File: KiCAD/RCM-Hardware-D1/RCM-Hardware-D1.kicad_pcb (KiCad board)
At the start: 2 copper layers, 66 x 63.5 mm, 2 parts, among them U1 WeMos_D1_mini, U2 L293D

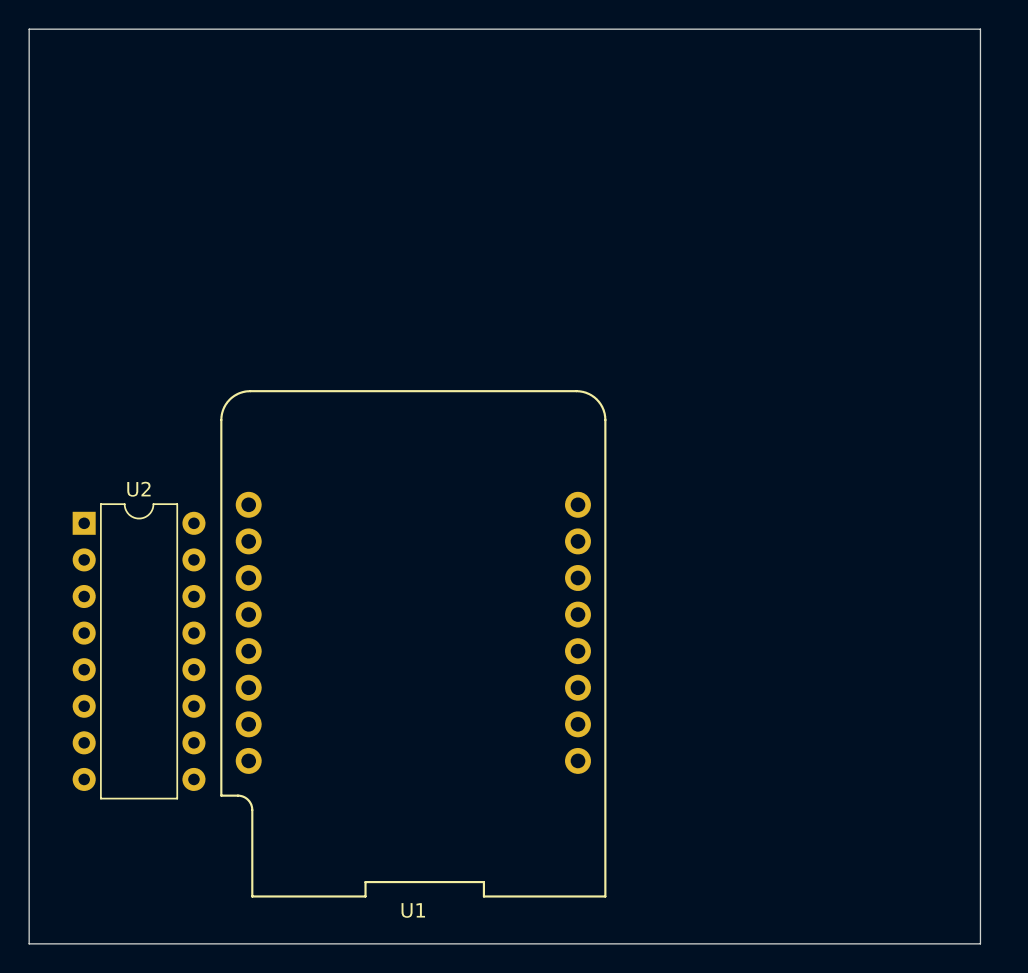
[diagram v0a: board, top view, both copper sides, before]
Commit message: Continued the KeyCAD for the circuit board
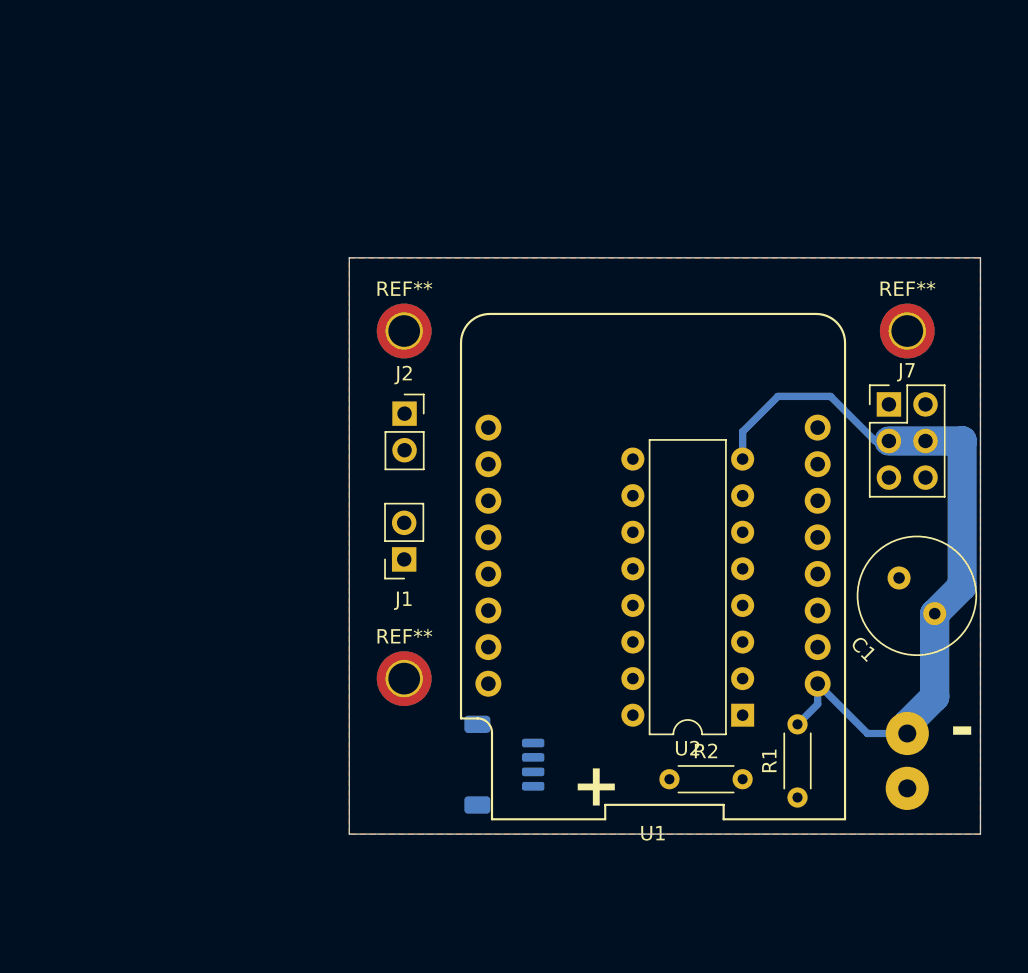
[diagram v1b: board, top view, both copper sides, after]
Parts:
- added C1: C_Polarized, Capacitor_THT:C_Radial_D8.0mm_H11.5mm_P3.50mm, F.Cu at (174.6, 83.8)
- added J1: Conn_01x02_Pin, Connector_PinSocket_2.54mm:PinSocket_1x02_P2.54mm_Vertical, F.Cu at (137.8, 80.0)
- added J2: Conn_01x02_Pin, Connector_PinSocket_2.54mm:PinSocket_1x02_P2.54mm_Vertical, F.Cu at (137.8, 69.9)
- added J3: battery, project:battery wires, F.Cu at (172.7, 92.1)
- added J6: Conn_01x04_Pin, Connector_JST:JST_SH_SM04B-SRSS-TB_1x04-1MP_P1.00mm_Horizontal, B.Cu at (144.8, 94.2)
- added J7: Conn_01x06_Pin, Connector_PinHeader_2.54mm:PinHeader_2x03_P2.54mm_Vertical, F.Cu at (171.4, 69.2)
- added R1: R, Resistor_THT:R_Axial_DIN0204_L3.6mm_D1.6mm_P5.08mm_Horizontal, F.Cu at (165.1, 96.5)
- added R2: R, Resistor_THT:R_Axial_DIN0204_L3.6mm_D1.6mm_P5.08mm_Horizontal, F.Cu at (156.2, 95.2)
- added REF**: MountingHole_2.2mm_M2_DIN965_Pad_TopBottom, MountingHole:MountingHole_2.2mm_M2_DIN965_Pad_TopBottom, F.Cu at (137.8, 88.3)
- added REF**: MountingHole_2.2mm_M2_DIN965_Pad_TopBottom, MountingHole:MountingHole_2.2mm_M2_DIN965_Pad_TopBottom, F.Cu at (137.8, 64.1)
- added REF**: MountingHole_2.2mm_M2_DIN965_Pad_TopBottom, MountingHole:MountingHole_2.2mm_M2_DIN965_Pad_TopBottom, F.Cu at (172.7, 64.1)
- moved U2 47.6 mm to (161.3, 90.8), turned to 180 degrees
- moved U1 17.5 mm to (155.1, 79.7)
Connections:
- U1 pad 13: unconnected-(U1-D2-Pad13) -> Net-(J6-Pin_3)
- U1 pad 14: unconnected-(U1-D1-Pad14) -> Net-(J6-Pin_4)
- U1 pad 2: unconnected-(U1-A0-Pad2) -> Net-(U1-A0)
- U1 pad 3: unconnected-(U1-D0-Pad3) -> Net-(U1-D0)
- U1 pad 4: unconnected-(U1-D5-Pad4) -> Net-(U1-D5)
- U1 pad 5: unconnected-(U1-D6-Pad5) -> Net-(U1-D6)
- U1 pad 6: unconnected-(U1-D7-Pad6) -> Net-(U1-D7)
- U1 pad 8: unconnected-(U1-3.3V-Pad8) -> +3.3V
- U1 pad 9: unconnected-(U1-5V-Pad9) -> Net-(J3-Pin_1)
- U2 pad 1: unconnected-(U2-EN1,2-Pad1) -> +3.3V
- U2 pad 10: unconnected-(U2-3A-Pad10) -> Net-(U1-D5)
- U2 pad 11: unconnected-(U2-3Y-Pad11) -> Net-(J1-Pin_2)
- U2 pad 14: unconnected-(U2-4Y-Pad14) -> Net-(J1-Pin_1)
- U2 pad 15: unconnected-(U2-4A-Pad15) -> Net-(U1-D6)
- U2 pad 16: unconnected-(U2-VCC1-Pad16) -> Net-(J3-Pin_1)
- U2 pad 2: unconnected-(U2-1A-Pad2) -> Net-(U1-D7)
- U2 pad 3: unconnected-(U2-1Y-Pad3) -> Net-(J2-Pin_2)
- U2 pad 6: unconnected-(U2-2Y-Pad6) -> Net-(J2-Pin_1)
- U2 pad 7: unconnected-(U2-2A-Pad7) -> Net-(U1-D0)
- U2 pad 8: unconnected-(U2-VCC2-Pad8) -> Net-(J3-Pin_1)
- U2 pad 9: unconnected-(U2-EN3,4-Pad9) -> +3.3V
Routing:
- net Net-(J3-Pin_1): track 0.00 -> 52.4 mm
- added copper zone on F.Cu, net GND
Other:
- board size 66 x 63.5 mm -> 43.8 x 40 mm
